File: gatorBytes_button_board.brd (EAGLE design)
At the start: 100.3 x 49.5 mm, 43 parts

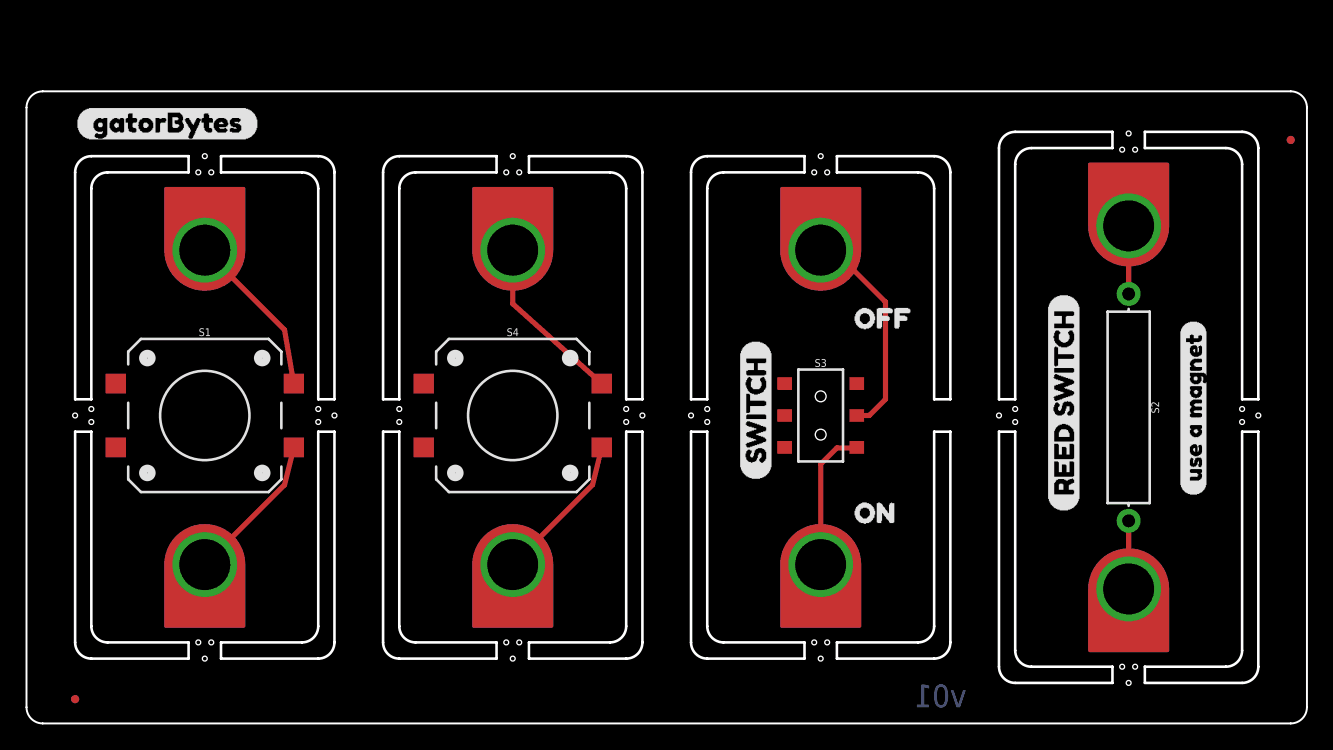
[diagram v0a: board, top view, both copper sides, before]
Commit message: pre design review
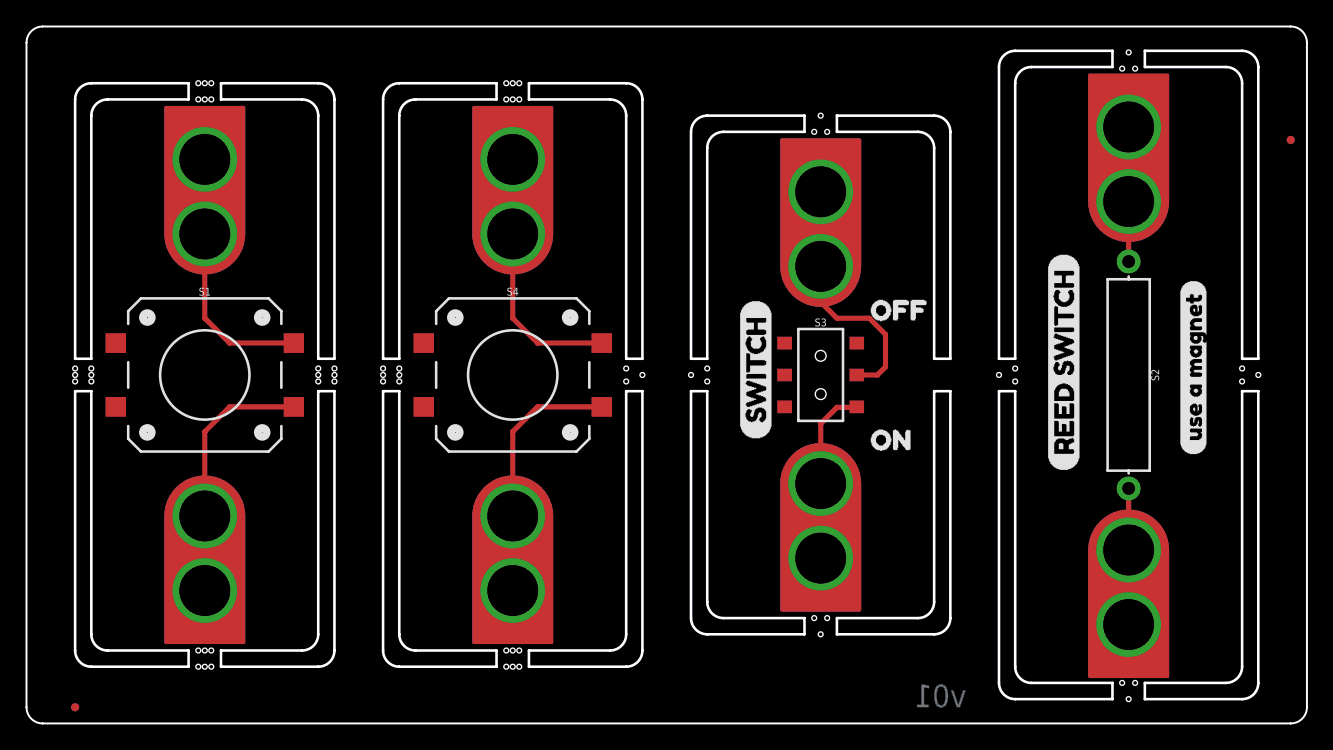
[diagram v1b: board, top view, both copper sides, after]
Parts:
- removed U$30: (no value), 003:GATORBYTES6
- U$10, U$11, U$12, U$14, U$15, U$16, U$17, U$19: value GATOR_MINI -> GATOR; device TAB:GATOR_MINI -> SparkFun-Connectors:GATOR
- moved U$14 11.4 mm to (62.2, 19.1)
- moved U$17 8.89 mm to (14.0, 16.5)
- moved U$19 8.89 mm to (38.1, 16.5)
- moved U$12 8.13 mm to (86.4, 13.8)
- moved LOGO7 6.35 mm to (80.6, 47.0)
- moved LOGO8 6.35 mm to (92.5, 48.1)
- moved U$15 6.35 mm to (62.2, 35.6)
- moved U$13 5.85 mm to (64.8, 22.2)
- moved LOGO4 5.72 mm to (32.4, 45.1)
- moved LOGO3 5.71 mm to (44.3, 46.4)
- moved LOGO5 5.71 mm to (20.2, 46.4)
- moved U$10 3.81 mm to (38.1, 38.1)
- moved U$11 3.81 mm to (14.0, 38.1)
- moved LOGO1 3.18 mm to (56.5, 42.5)
- moved S1 3.18 mm to (14.0, 27.3)
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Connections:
- net N$1: now also U$19.P$1, U$19.P$2; no longer U$19.P1
- net N$2: now also U$10.P$1, U$10.P$2; no longer U$10.P1
- net N$3: now also U$17.P$1, U$17.P$2; no longer U$17.P1
- net N$4: now also U$11.P$1, U$11.P$2; no longer U$11.P1
- net N$5: now also U$16.P$1, U$16.P$2; no longer U$16.P1
- net N$6: now also U$12.P$1, U$12.P$2; no longer U$12.P1
- net N$7: now also U$15.P$1, U$15.P$2; no longer U$15.P1
- net N$9: now also U$14.P$1, U$14.P$2; no longer U$14.P1
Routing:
- net N$5: track 5.33 -> 11.8 mm
- net N$6: track 5.33 -> 10.7 mm
- net N$9: track 11.2 -> 13.9 mm
- net N$3: track 11.9 -> 14.4 mm
- net N$1: track 11.9 -> 14.4 mm
- net N$2: track 13.6 -> 15.8 mm
- net N$4: track 13.1 -> 14.4 mm
- net N$7: track 18.7 -> 17.7 mm
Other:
- board size 100.3 x 49.5 mm -> 100.3 x 54.6 mm
